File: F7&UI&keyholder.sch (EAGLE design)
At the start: 27 parts, among them IC2 LTC485N, IC4 MCP2561-E_P

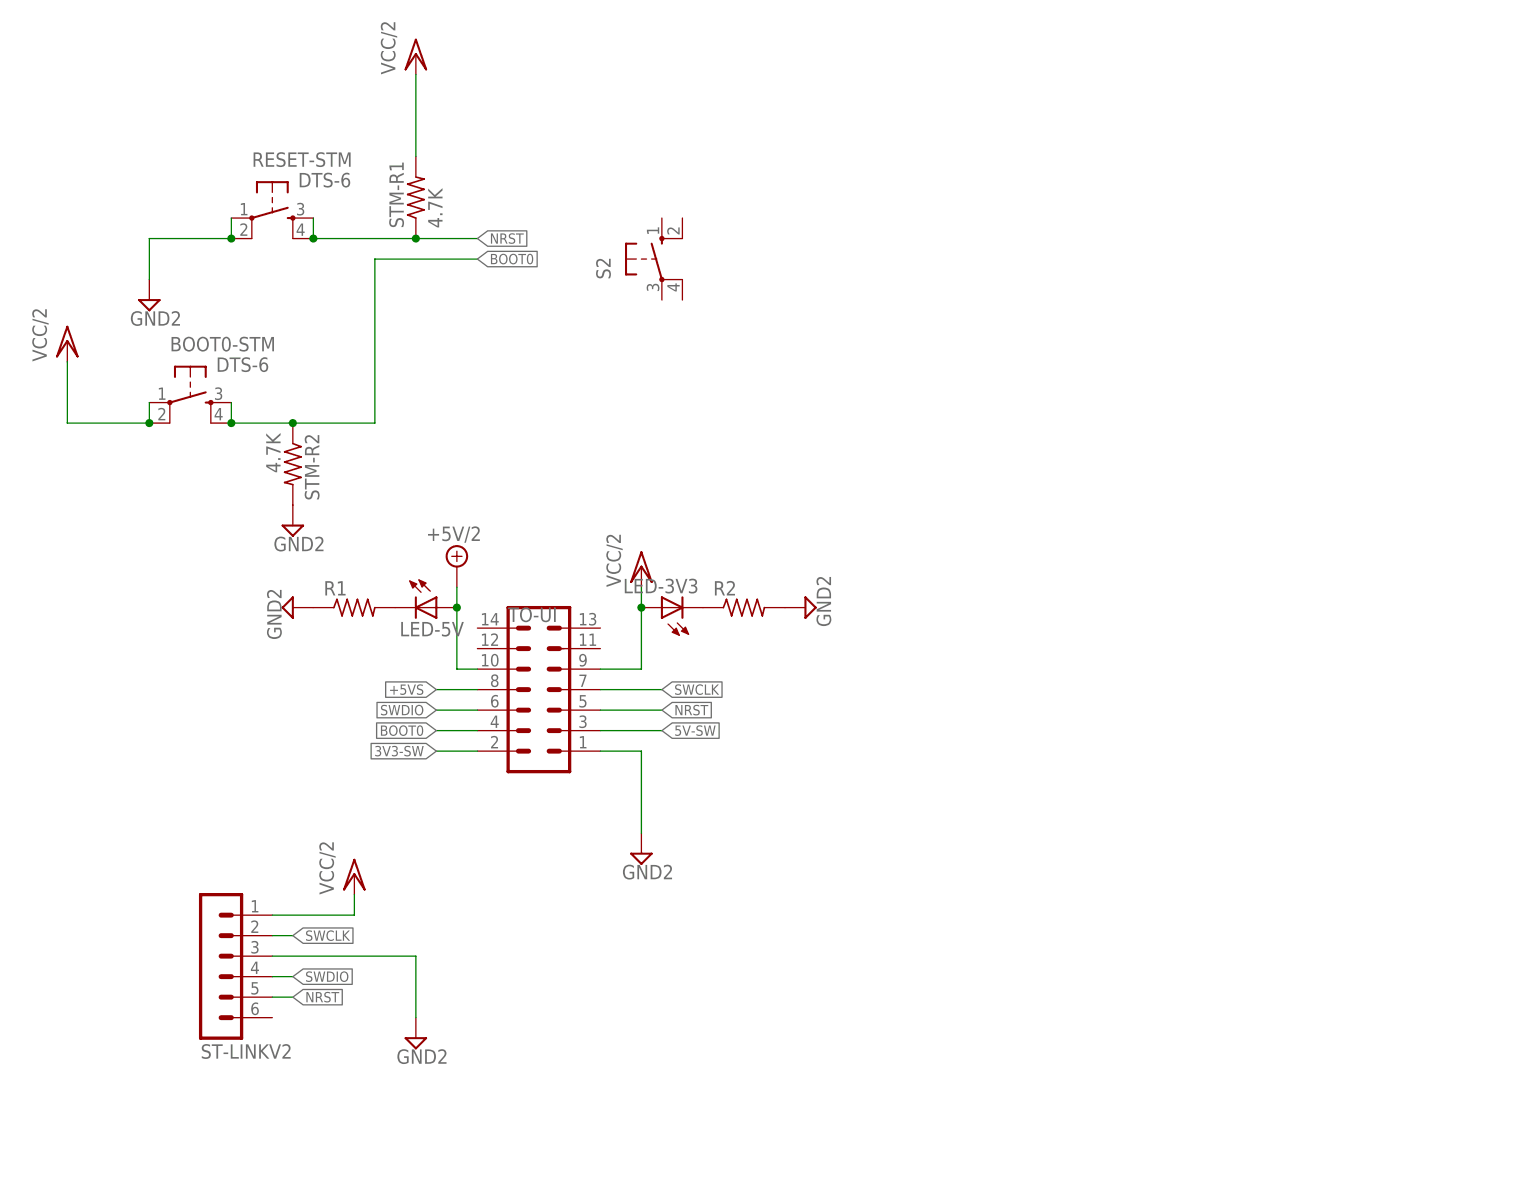
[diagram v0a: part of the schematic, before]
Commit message: #OTL 意外とやること多い
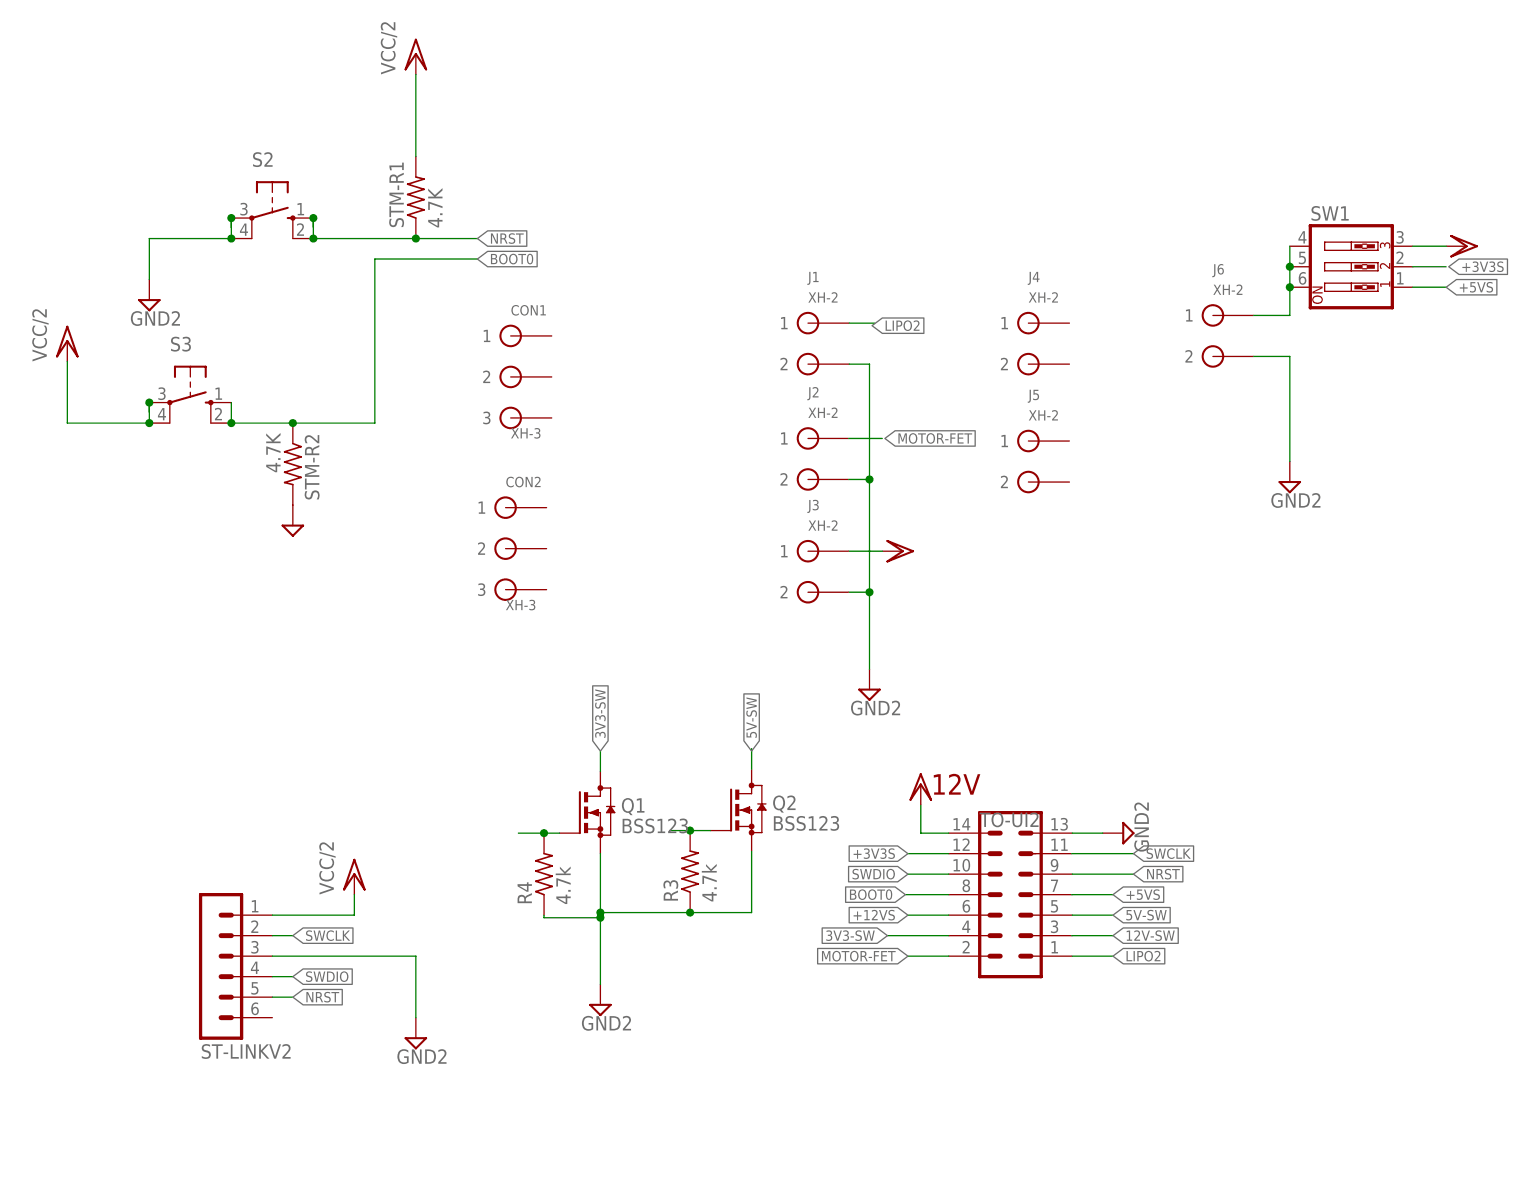
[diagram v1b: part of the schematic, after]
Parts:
- removed BOOT0-STM, RESET-STM: DTS-6, forprint:DTS-6
- removed LED-3V3, LED-5V: (no value), adafruit:LED5MM
- removed R1, R2: (no value), resistor:R-US_M0805
- removed TO-UI: (no value), 0con-harting-ml:ML14
- added CON1, CON2: XH-3, 0@Mylibrary-main1:XH-3
- added J1, J2, J3, J4, J5, J6: XH-2, 0@Mylibrary-main1:XH-2
- added Q1, Q2: BSS123, transistor-small-signal:BSS123
- added R3, R4: 4.7k, resistor:R-US_M0805
- added S3: (no value), switch-omron:40-XX
- added SW1: (no value), special:SW_DIP-3
- added TO-UI2: (no value), 0con-harting-ml:ML14
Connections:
- removed net +5V/2: LED-5V.A, TO-UI.10
- removed net N$7: LED-5V.C, R1.2
- removed net N$8: LED-3V3.C, R2.1
- new net +12VS: TO-UI2.6
- new net +3V3S: SW1.2, TO-UI2.12
- new net 12V-SW: TO-UI2.3
- new net LIPO2: J1.1, TO-UI2.1
- new net MOTOR-FET: J2.1, TO-UI2.2
- new net N$2: Q1.G, R4.2
- new net N$3: Q2.G, R3.2
- new net N$6: J6.1, SW1.4, SW1.5, SW1.6
- new net VDD: J3.1, SW1.3, TO-UI2.14
- net +5VS: now also SW1.1, TO-UI2.7; no longer TO-UI.8
- net 3V3-SW: now also Q1.D, TO-UI2.4; no longer TO-UI.2
- net 5V-SW: now also Q2.D, TO-UI2.5; no longer TO-UI.3
- net BOOT0: now also S3.S, S3.S1, TO-UI2.8; no longer BOOT0-STM.3, BOOT0-STM.4, TO-UI.4
- net GND2: now also J1.2, J2.2, J3.2, J6.2, Q1.S, Q2.S, R3.1, R4.1, S2.P, S2.P1, TO-UI2.13; no longer R1.1, R2.2, RESET-STM.1, RESET-STM.2, TO-UI.1
- net NRST: now also S2.S, S2.S1, TO-UI2.9; no longer RESET-STM.3, RESET-STM.4, TO-UI.5
- net SWCLK: now also TO-UI2.11; no longer TO-UI.7
- net SWDIO: now also TO-UI2.10; no longer TO-UI.6
- net VCC/2: now also S3.P, S3.P1; no longer BOOT0-STM.1, BOOT0-STM.2, LED-3V3.A, TO-UI.9
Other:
- note added: "12V"
- moved on the sheet: S2
